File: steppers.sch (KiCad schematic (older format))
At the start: 30 parts, among them J1 Conn_02x03_Odd_Even, J10 Conn_01x04, J2 Conn_02x03_Odd_Even, J3 Conn_01x04, J4 Conn_01x04, J5 Conn_02x03_Odd_Even, J6 Conn_02x03_Odd_Even, J7 Conn_01x04, J8 Conn_01x04, J9 Conn_02x03_Odd_Even

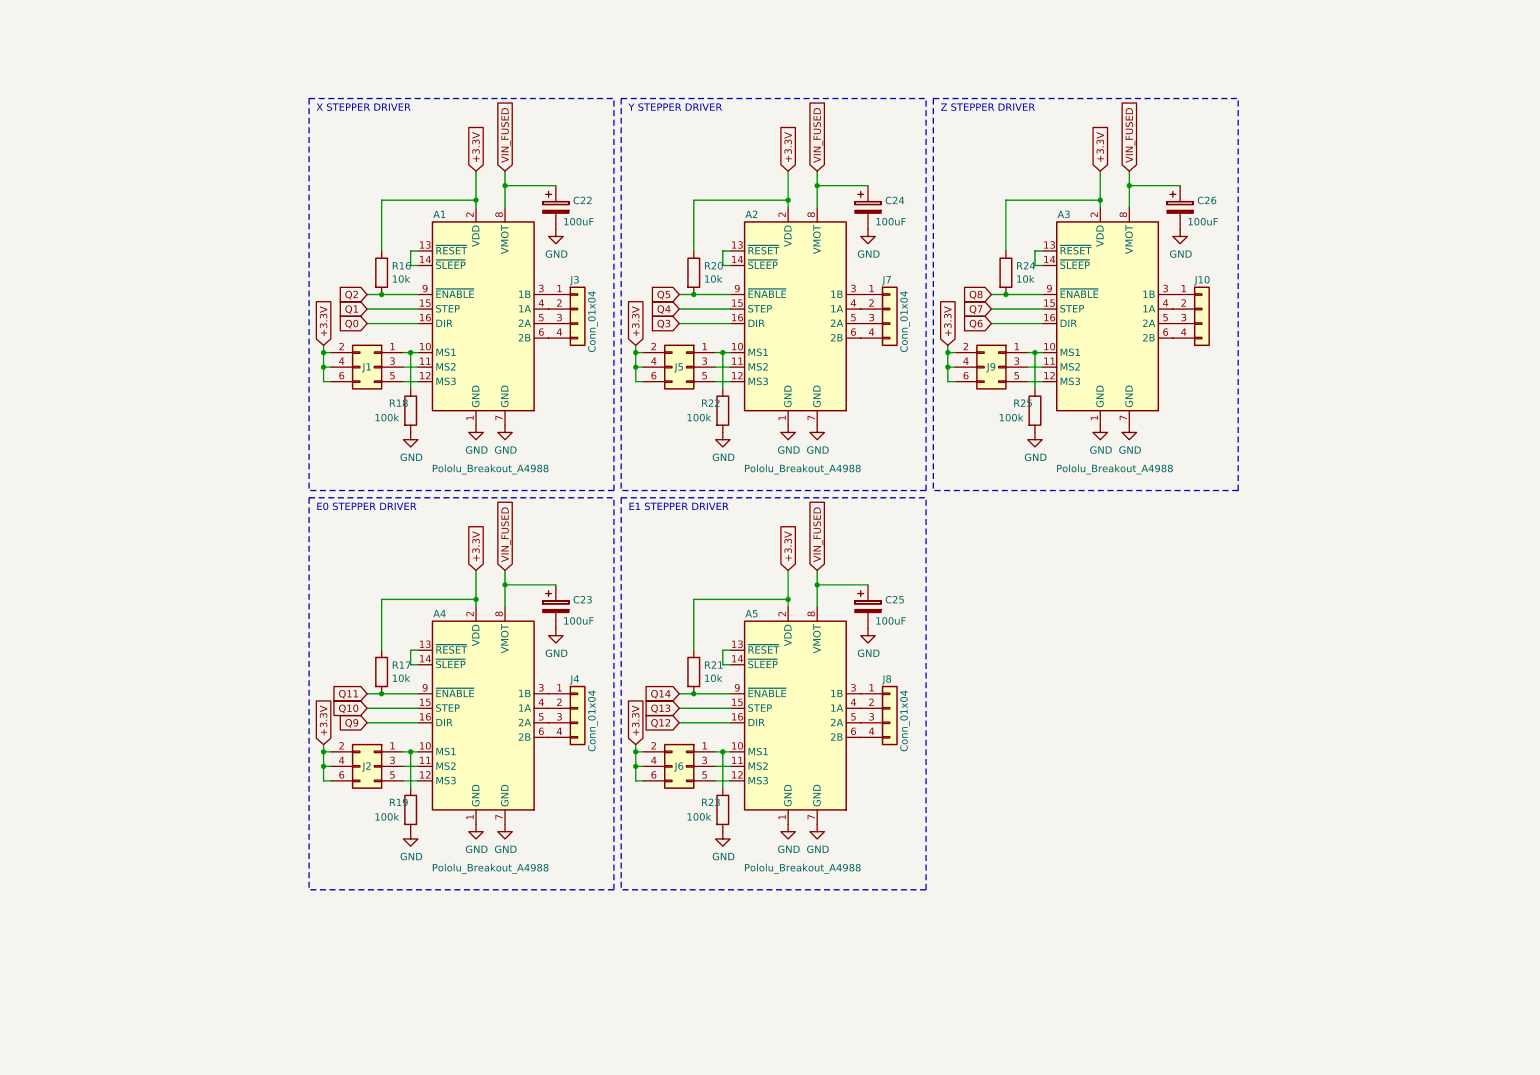
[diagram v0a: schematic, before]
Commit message: Prototype R3
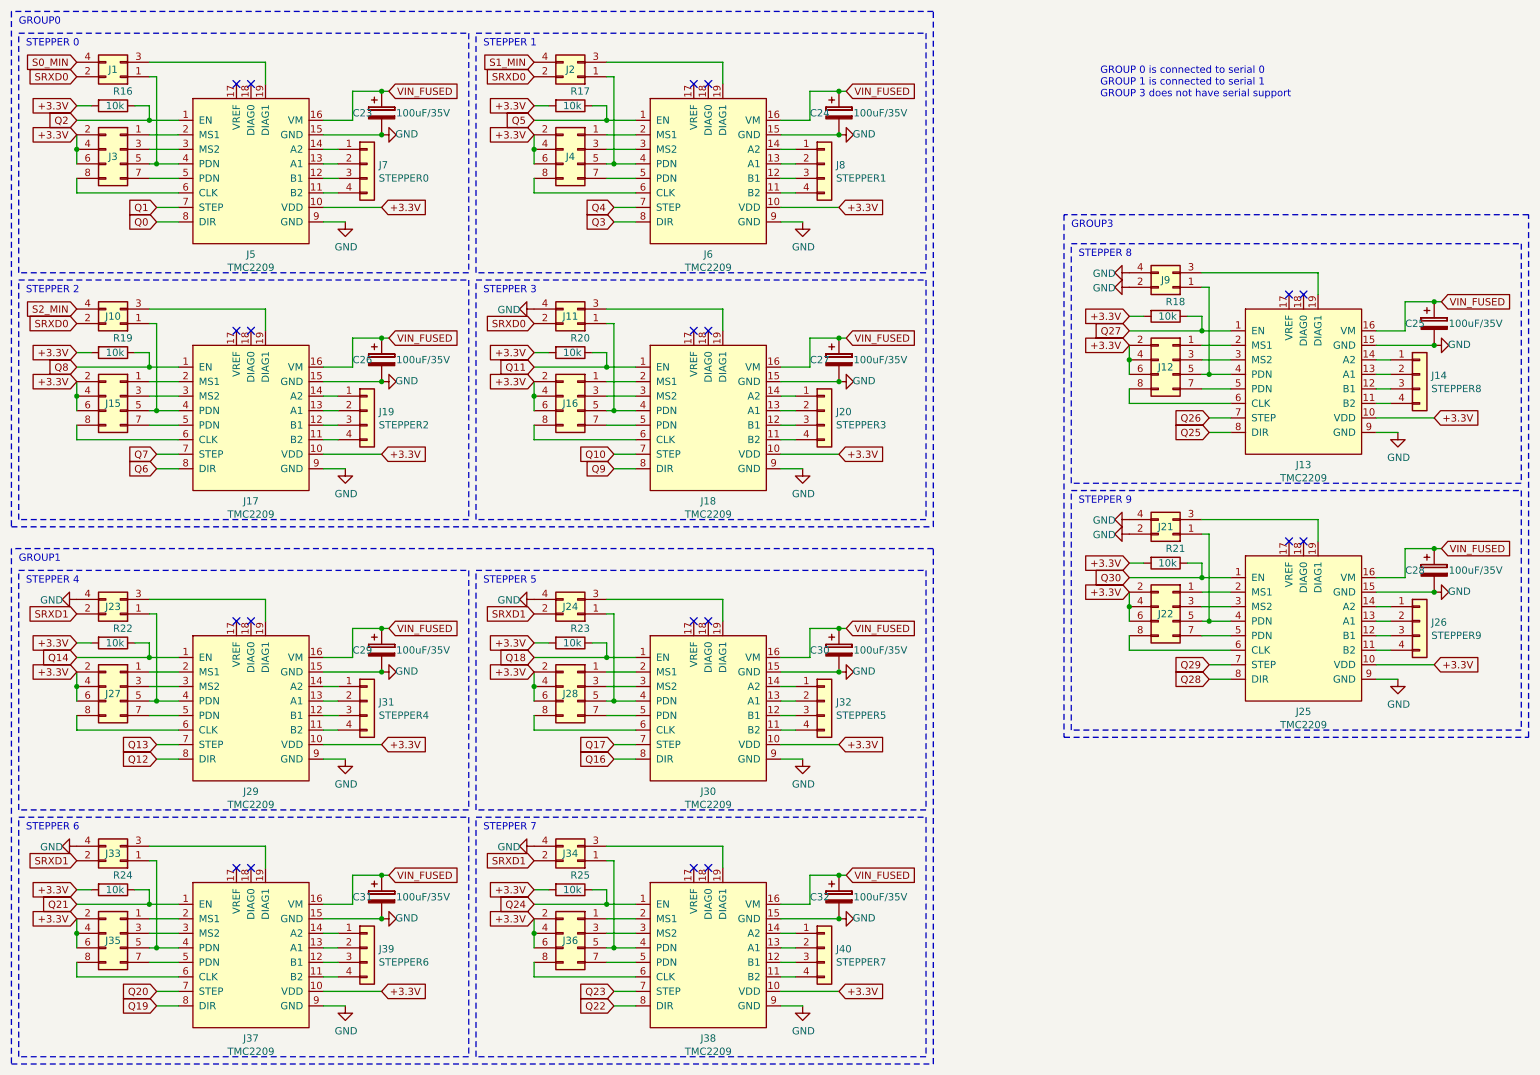
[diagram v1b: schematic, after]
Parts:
- removed A1, A2, A3, A4, A5: Pololu_Breakout_A4988, Module:Pololu_Breakout-16_15.2x20.3mm, symbol esp32controller-rescue:Pololu_Breakout_A4988-Driver_Motor
- removed C22: 100uF, Capacitor_SMD:CP_Elec_6.3x7.7, symbol esp32controller-rescue:CP-Device
- removed J1, J2, J5, J6, J9: Conn_02x03_Odd_Even, Connector_PinHeader_2.54mm:PinHeader_2x03_P2.54mm_Vertical, symbol esp32controller-rescue:Conn_02x03_Odd_Even-Connector_Generic
- removed J10, J3, J4, J7, J8: Conn_01x04, ESP32Controller:Socket_Strip_Straight_1x04_Pitch2.54mm_dual, symbol esp32controller-rescue:Conn_01x04-Connector_Generic
- added C27, C28, C29, C30, C31, C32: 100uF/35V, Capacitor_SMD:CP_Elec_6.3x7.7, symbol esp32controller-rescue:CP-Device
- added J1, J10, J11, J2, J21, J23, J24, J33, J34, J9: Conn_02x02_Odd_Even, Connector_PinHeader_2.54mm:PinHeader_1x04_P2.54mm_Vertical, symbol Connector_Generic:Conn_02x02_Odd_Even
- added J12, J15, J16, J22, J27, J28, J3, J35, J36, J4: Conn_02x04_Odd_Even, Connector_PinHeader_2.54mm:PinHeader_2x04_P2.54mm_Vertical, symbol Connector_Generic:Conn_02x04_Odd_Even
- added J13, J17, J18, J25, J29, J30, J37, J38, J5, J6: TMC2209, ESP32Controller:pololu, symbol ESP32Controller:TMC2209
- added J14: STEPPER8, Connector_JST:JST_XH_B4B-XH-A_1x04_P2.50mm_Vertical, symbol Connector_Generic:Conn_01x04
- added J19: STEPPER2, Connector_JST:JST_XH_B4B-XH-A_1x04_P2.50mm_Vertical, symbol Connector_Generic:Conn_01x04
- added J20: STEPPER3, Connector_JST:JST_XH_B4B-XH-A_1x04_P2.50mm_Vertical, symbol Connector_Generic:Conn_01x04
- added J26: STEPPER9, Connector_JST:JST_XH_B4B-XH-A_1x04_P2.50mm_Vertical, symbol Connector_Generic:Conn_01x04
- added J31: STEPPER4, Connector_JST:JST_XH_B4B-XH-A_1x04_P2.50mm_Vertical, symbol Connector_Generic:Conn_01x04
- added J32: STEPPER5, Connector_JST:JST_XH_B4B-XH-A_1x04_P2.50mm_Vertical, symbol Connector_Generic:Conn_01x04
- added J39: STEPPER6, Connector_JST:JST_XH_B4B-XH-A_1x04_P2.50mm_Vertical, symbol Connector_Generic:Conn_01x04
- added J40: STEPPER7, Connector_JST:JST_XH_B4B-XH-A_1x04_P2.50mm_Vertical, symbol Connector_Generic:Conn_01x04
- added J7: STEPPER0, Connector_JST:JST_XH_B4B-XH-A_1x04_P2.50mm_Vertical, symbol Connector_Generic:Conn_01x04
- added J8: STEPPER1, Connector_JST:JST_XH_B4B-XH-A_1x04_P2.50mm_Vertical, symbol Connector_Generic:Conn_01x04
- C23, C24, C25, C26: value 100uF -> 100uF/35V
- R18, R19, R22, R23, R25: value 100k -> 10k
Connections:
- net +3.3V: now also R16.2, R17.2, R18.2, R19.2, R20.2, R21.2, R22.2, R23.2, R24.2, R25.2, J12.2 (Pin_2), J12.4 (Pin_4), J12.6 (Pin_6), J13.10 (VDD), J15.2 (Pin_2), J15.4 (Pin_4), J15.6 (Pin_6), J16.2 (Pin_2), J16.4 (Pin_4), J16.6 (Pin_6), J17.10 (VDD), J18.10 (VDD), J22.2 (Pin_2), J22.4 (Pin_4), J22.6 (Pin_6), J25.10 (VDD), J27.2 (Pin_2), J27.4 (Pin_4), J27.6 (Pin_6), J28.2 (Pin_2), J28.4 (Pin_4), J28.6 (Pin_6), J29.10 (VDD), J3.2 (Pin_2), J3.4 (Pin_4), J3.6 (Pin_6), J30.10 (VDD), J35.2 (Pin_2), J35.4 (Pin_4), J35.6 (Pin_6), J36.2 (Pin_2), J36.4 (Pin_4), J36.6 (Pin_6), J37.10 (VDD), J38.10 (VDD), J4.2 (Pin_2), J4.4 (Pin_4), J4.6 (Pin_6), J5.10 (VDD), J6.10 (VDD); no longer R16.1, R17.1, R20.1, R21.1, R24.1
- net GND: now also C27.2, C28.2, C29.2, C30.2, C31.2, C32.2, J11.4 (Pin_4), J13.15 (GND), J13.9 (GND), J17.15 (GND), J17.9 (GND), J18.15 (GND), J18.9 (GND), J21.2 (Pin_2), J21.4 (Pin_4), J23.4 (Pin_4), J24.4 (Pin_4), J25.15 (GND), J25.9 (GND), J29.15 (GND), J29.9 (GND), J30.15 (GND), J30.9 (GND), J33.4 (Pin_4), J34.4 (Pin_4), J37.15 (GND), J37.9 (GND), J38.15 (GND), J38.9 (GND), J5.15 (GND), J5.9 (GND), J6.15 (GND), J6.9 (GND), J9.2 (Pin_2), J9.4 (Pin_4); no longer R18.2, R19.2, R22.2, R23.2, R25.2
- net Q0: now also J5.8 (DIR)
- net Q1: now also J5.7 (STEP)
- net Q10: now also J18.7 (STEP)
- net Q11: now also R20.1, J18.1 (EN); no longer R17.2
- net Q12: now also J29.8 (DIR)
- net Q13: now also J29.7 (STEP)
- net Q14: now also R22.1, J29.1 (EN); no longer R21.2
- net Q2: now also R16.1, J5.1 (EN); no longer R16.2
- net Q3: now also J6.8 (DIR)
- net Q4: now also J6.7 (STEP)
- net Q5: now also R17.1, J6.1 (EN); no longer R20.2
- net Q6: now also J17.8 (DIR)
- net Q7: now also J17.7 (STEP)
- net Q8: now also R19.1, J17.1 (EN); no longer R24.2
- net Q9: now also J18.8 (DIR)
- net VIN_FUSED: now also C27.1, C28.1, C29.1, C30.1, C31.1, C32.1, J13.16 (VM), J17.16 (VM), J18.16 (VM), J25.16 (VM), J29.16 (VM), J30.16 (VM), J37.16 (VM), J38.16 (VM), J5.16 (VM), J6.16 (VM)
- net Q27: now reaches R18.1
- net Q27: now also J13.1 (EN)
- net Q24: now reaches R25.1
- net Q24: now also J38.1 (EN)
- net Q18: now reaches R23.1
- net Q18: now also J30.1 (EN)
- new net: J5.11 (B2), J7.4 (Pin_4)
- new net: J5.12 (B1), J7.3 (Pin_3)
- new net: J5.13 (A1), J7.2 (Pin_2)
- new net: J5.14 (A2), J7.1 (Pin_1)
- new net: J1.3 (Pin_3), J5.19 (DIAG1)
- new net: J3.1 (Pin_1), J5.2 (MS1)
- new net: J3.3 (Pin_3), J5.3 (MS2)
- new net: J1.1 (Pin_1), J3.5 (Pin_5), J5.4 (PDN)
- new net: J3.7 (Pin_7), J5.5 (PDN)
- new net: J3.8 (Pin_8), J5.6 (CLK)
- new net: J6.11 (B2), J8.4 (Pin_4)
- new net: J6.12 (B1), J8.3 (Pin_3)
- new net: J6.13 (A1), J8.2 (Pin_2)
- new net: J6.14 (A2), J8.1 (Pin_1)
- new net: J2.3 (Pin_3), J6.19 (DIAG1)
- new net: J4.1 (Pin_1), J6.2 (MS1)
- new net: J4.3 (Pin_3), J6.3 (MS2)
- new net: J2.1 (Pin_1), J4.5 (Pin_5), J6.4 (PDN)
- new net: J4.7 (Pin_7), J6.5 (PDN)
- new net: J4.8 (Pin_8), J6.6 (CLK)
- new net: J13.11 (B2), J14.4 (Pin_4)
- new net: J13.12 (B1), J14.3 (Pin_3)
- new net: J13.13 (A1), J14.2 (Pin_2)
- new net: J13.14 (A2), J14.1 (Pin_1)
- new net: J13.19 (DIAG1), J9.3 (Pin_3)
- new net: J12.1 (Pin_1), J13.2 (MS1)
- new net: J12.3 (Pin_3), J13.3 (MS2)
- new net: J12.5 (Pin_5), J13.4 (PDN), J9.1 (Pin_1)
- new net: J12.7 (Pin_7), J13.5 (PDN)
- new net: J12.8 (Pin_8), J13.6 (CLK)
- new net: J17.11 (B2), J19.4 (Pin_4)
- new net: J17.12 (B1), J19.3 (Pin_3)
- new net: J17.13 (A1), J19.2 (Pin_2)
- new net: J17.14 (A2), J19.1 (Pin_1)
- new net: J10.3 (Pin_3), J17.19 (DIAG1)
- new net: J15.1 (Pin_1), J17.2 (MS1)
- new net: J15.3 (Pin_3), J17.3 (MS2)
- new net: J10.1 (Pin_1), J15.5 (Pin_5), J17.4 (PDN)
- new net: J15.7 (Pin_7), J17.5 (PDN)
- new net: J15.8 (Pin_8), J17.6 (CLK)
- new net: J18.11 (B2), J20.4 (Pin_4)
- new net: J18.12 (B1), J20.3 (Pin_3)
- new net: J18.13 (A1), J20.2 (Pin_2)
- new net: J18.14 (A2), J20.1 (Pin_1)
- new net: J11.3 (Pin_3), J18.19 (DIAG1)
- new net: J16.1 (Pin_1), J18.2 (MS1)
- new net: J16.3 (Pin_3), J18.3 (MS2)
- new net: J11.1 (Pin_1), J16.5 (Pin_5), J18.4 (PDN)
- new net: J16.7 (Pin_7), J18.5 (PDN)
- new net: J16.8 (Pin_8), J18.6 (CLK)
- new net: J25.11 (B2), J26.4 (Pin_4)
- new net: J25.12 (B1), J26.3 (Pin_3)
- new net: J25.13 (A1), J26.2 (Pin_2)
- new net: J25.14 (A2), J26.1 (Pin_1)
- new net: J21.3 (Pin_3), J25.19 (DIAG1)
- new net: J22.1 (Pin_1), J25.2 (MS1)
- new net: J22.3 (Pin_3), J25.3 (MS2)
- new net: J21.1 (Pin_1), J22.5 (Pin_5), J25.4 (PDN)
- new net: J22.7 (Pin_7), J25.5 (PDN)
- new net: J22.8 (Pin_8), J25.6 (CLK)
- new net: J29.11 (B2), J31.4 (Pin_4)
- new net: J29.12 (B1), J31.3 (Pin_3)
- new net: J29.13 (A1), J31.2 (Pin_2)
- new net: J29.14 (A2), J31.1 (Pin_1)
- new net: J23.3 (Pin_3), J29.19 (DIAG1)
- new net: J27.1 (Pin_1), J29.2 (MS1)
- new net: J27.3 (Pin_3), J29.3 (MS2)
- new net: J23.1 (Pin_1), J27.5 (Pin_5), J29.4 (PDN)
- new net: J27.7 (Pin_7), J29.5 (PDN)
- new net: J27.8 (Pin_8), J29.6 (CLK)
- new net: J30.11 (B2), J32.4 (Pin_4)
- new net: J30.12 (B1), J32.3 (Pin_3)
- new net: J30.13 (A1), J32.2 (Pin_2)
- new net: J30.14 (A2), J32.1 (Pin_1)
- new net: J24.3 (Pin_3), J30.19 (DIAG1)
- new net: J28.1 (Pin_1), J30.2 (MS1)
- new net: J28.3 (Pin_3), J30.3 (MS2)
- new net: J24.1 (Pin_1), J28.5 (Pin_5), J30.4 (PDN)
- new net: J28.7 (Pin_7), J30.5 (PDN)
- new net: J28.8 (Pin_8), J30.6 (CLK)
- new net: J37.11 (B2), J39.4 (Pin_4)
- new net: J37.12 (B1), J39.3 (Pin_3)
- new net: J37.13 (A1), J39.2 (Pin_2)
- new net: J37.14 (A2), J39.1 (Pin_1)
- new net: J33.3 (Pin_3), J37.19 (DIAG1)
- new net: J35.1 (Pin_1), J37.2 (MS1)
- new net: J35.3 (Pin_3), J37.3 (MS2)
- new net: J33.1 (Pin_1), J35.5 (Pin_5), J37.4 (PDN)
- new net: J35.7 (Pin_7), J37.5 (PDN)
- new net: J35.8 (Pin_8), J37.6 (CLK)
- new net: J38.11 (B2), J40.4 (Pin_4)
- new net: J38.12 (B1), J40.3 (Pin_3)
- new net: J38.13 (A1), J40.2 (Pin_2)
- new net: J38.14 (A2), J40.1 (Pin_1)
- new net: J34.3 (Pin_3), J38.19 (DIAG1)
- new net: J36.1 (Pin_1), J38.2 (MS1)
- new net: J36.3 (Pin_3), J38.3 (MS2)
- new net: J34.1 (Pin_1), J36.5 (Pin_5), J38.4 (PDN)
- new net: J36.7 (Pin_7), J38.5 (PDN)
- new net: J36.8 (Pin_8), J38.6 (CLK)
- new net Q16: J30.8 (DIR)
- new net Q17: J30.7 (STEP)
- new net Q19: J37.8 (DIR)
- new net Q20: J37.7 (STEP)
- new net Q21: J37.1 (EN), R24.1
- new net Q22: J38.8 (DIR)
- new net Q23: J38.7 (STEP)
- new net Q25: J13.8 (DIR)
- new net Q26: J13.7 (STEP)
- new net Q28: J25.8 (DIR)
- new net Q29: J25.7 (STEP)
- new net Q30: J25.1 (EN), R21.1
- new net S0_MIN: J1.4 (Pin_4)
- new net S1_MIN: J2.4 (Pin_4)
- new net S2_MIN: J10.4 (Pin_4)
- new net SRXD0: J1.2 (Pin_2), J10.2 (Pin_2), J11.2 (Pin_2), J2.2 (Pin_2)
- new net SRXD1: J23.2 (Pin_2), J24.2 (Pin_2), J33.2 (Pin_2), J34.2 (Pin_2)
- no-connect marks 0 -> 20
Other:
- note added: "GROUP 0 is connected to serial 0\nGROUP 1 is connected to serial 1\nGROUP 3 does not have serial support"
- note added: "GROUP0"
- note added: "GROUP1"
- note added: "GROUP3"
- note added: "STEPPER 0"
- note added: "STEPPER 1"
- note added: "STEPPER 2"
- note added: "STEPPER 3"
- note added: "STEPPER 4"
- note added: "STEPPER 5"
- note added: "STEPPER 6"
- note added: "STEPPER 7"
- note added: "STEPPER 8"
- note added: "STEPPER 9"
- note removed: "E0 STEPPER DRIVER"
- note removed: "E1 STEPPER DRIVER"
- note removed: "X STEPPER DRIVER"
- note removed: "Y STEPPER DRIVER"
- note removed: "Z STEPPER DRIVER"
